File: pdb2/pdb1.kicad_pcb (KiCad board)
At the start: 2 copper layers, 99.1 x 17.8 mm, 24 parts, among them P1 CONN_XT60, P2 CONN_XT60, P3 CONN_02X03, P4 CONN_01X02, P5 CONN_01X02, Q2 BUK9Y4R8-60E, U1 INA169, U2 NSI45020AT1G, U3 NSI45020AT1G, U4 LM3480-3.3, U5 74LVC1G08, U7 MIC5014, U8 NSI45020AT1G

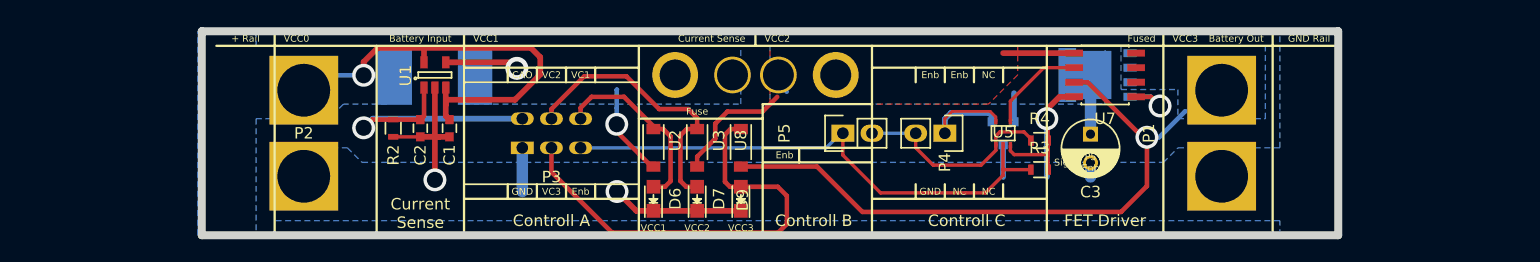
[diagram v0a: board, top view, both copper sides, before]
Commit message: test
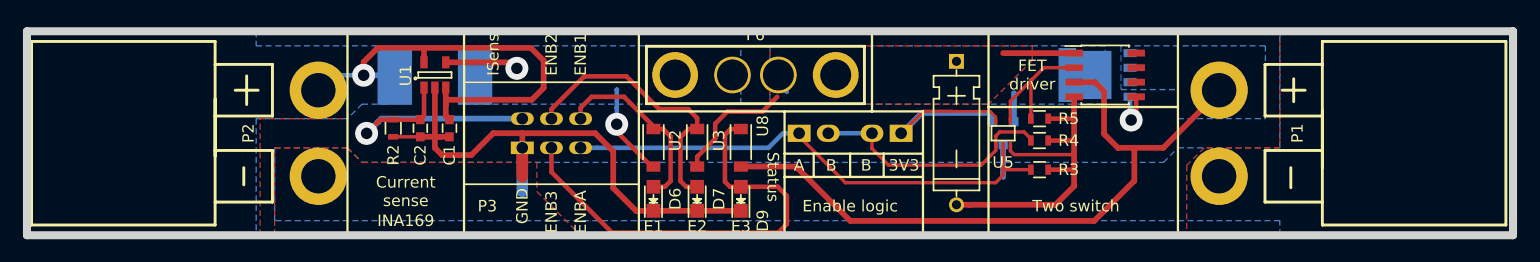
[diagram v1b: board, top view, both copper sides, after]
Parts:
- added R5: R, Resistors_SMD:R_0603, F.Cu at (123.8, 58.4)
- C3: footprint Capacitors_ThroughHole:C_Radial_D5_L6_P2.5 -> KiCad-Dev:C_Axial_D5_Custom
- F6: moved to F.Cu
- P1: footprint KiCad-Dev:XT60 -> KiCad-Dev:XT60_Horizontal1
- P2: footprint KiCad-Dev:XT60 -> KiCad-Dev:XT60_Horizontal2
- moved P1 17.8 mm to (157.5, 59.7)
- moved P2 16.7 mm to (43.0, 59.7), turned to 270 degrees
- moved C3 14.8 mm to (116.6, 50.7)
- moved P5 3.81 mm to (102.9, 59.7)
- moved P4 3.81 mm to (111.8, 59.7)
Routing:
- net /channel/GND: track 50.7 -> 84.7 mm, vias 3 -> 0
- net Net-(P4-Pad1): track 12.8 -> 18.9 mm
- net /channel/out+: track 54.8 -> 60.6 mm, vias 1 -> 0
- net /channel/kill_sw/in+: track 29.3 -> 24.3 mm
- net Net-(P4-Pad2): track 18.1 -> 21.9 mm
- net Net-(R5-Pad1): track 8.55 -> 12.0 mm
- net /channel/kill_sw/enable: track 46.3 -> 44.6 mm
- net Net-(Q2-Pad4): track 5.37 -> 4.26 mm
- net /channel/in+: track 40.7 -> 41.9 mm
- added copper zone on F.Cu, net /channel/GND
- added copper zone on F.Cu, net /channel/in+
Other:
- board size 99.1 x 17.8 mm -> 129.5 x 17.8 mm
- board text added: "2016-11-18 Version 1 jam12003@ student.mdh.se"
- board text added: "3V3"
- board text added: "A"
- board text added: "B"
- board text added: "Current sense"
- board text added: "E1"
- board text added: "E2"
- board text added: "E3"
- board text added: "ENB1"
- board text added: "ENB2"
- board text added: "ENB3"
- board text added: "ENBA"
- board text added: "Enable logic"
- board text added: "FET driver"
- board text added: "INA169"
- board text added: "ISens"
- board text added: "NAIAD"
- board text added: "Status"
- board text added: "Two switch"
- board text removed: "+ Rail"
- board text removed: "Battery Input"
- board text removed: "Battery Out"
- board text removed: "CAO"
- board text removed: "Controll A"
- board text removed: "Controll B"
- board text removed: "Controll C"
- board text removed: "Current Sense"
- board text removed: "Enb"
- board text removed: "FET Driver"
- board text removed: "Fuse"
- board text removed: "Fused"
- board text removed: "GND Rail"
- board text removed: "NC"
- board text removed: "P5 Enb"
- board text removed: "Sig"
- board text removed: "VC1"
- board text removed: "VC2"
- board text removed: "VC3"
- board text removed: "VCC0"
- board text removed: "VCC1"
- board text removed: "VCC2"
- board text removed: "VCC3"
